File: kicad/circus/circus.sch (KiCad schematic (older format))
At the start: 119 parts, among them Q4 2N4093, Q5 2N4093, U6 MM5837, U8 LM348

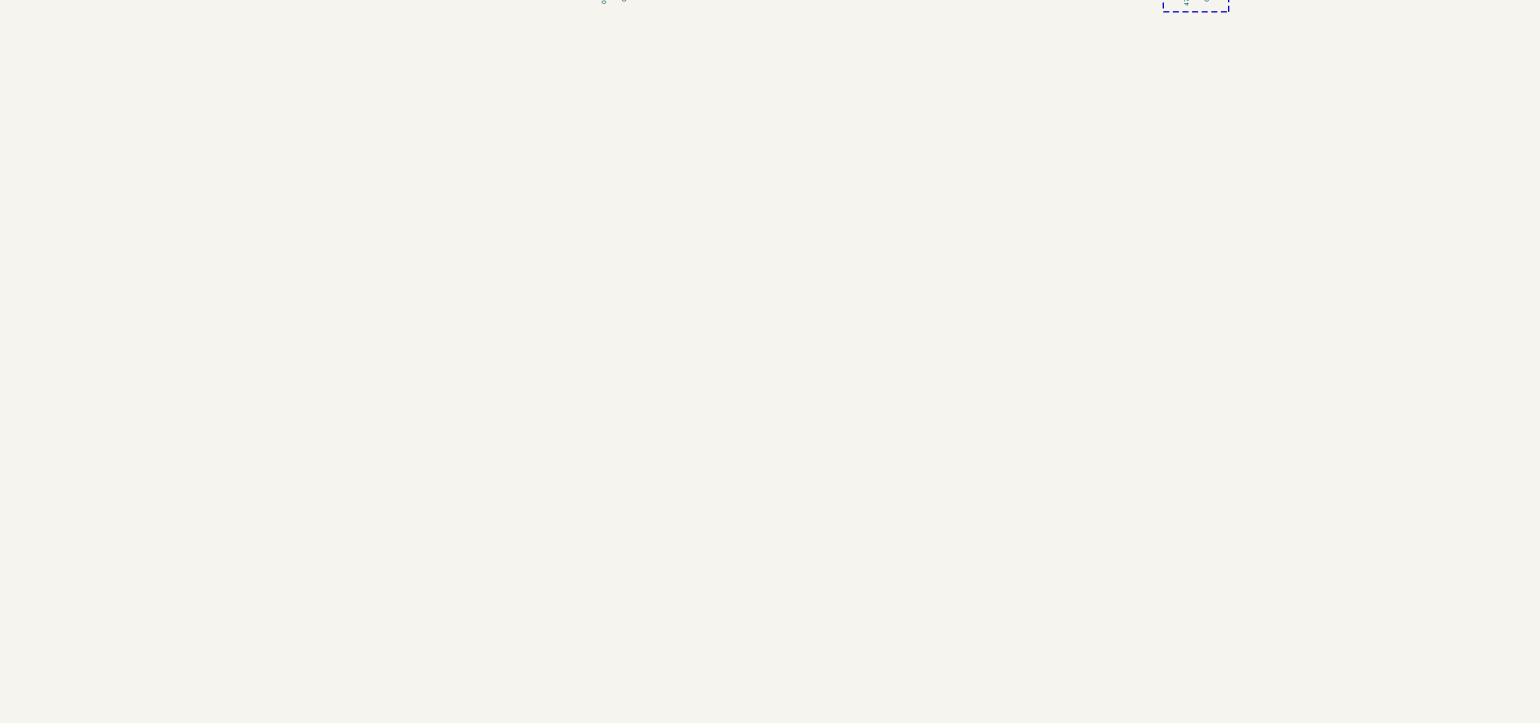
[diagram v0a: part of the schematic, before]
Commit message: The bear sound is now half-complete.
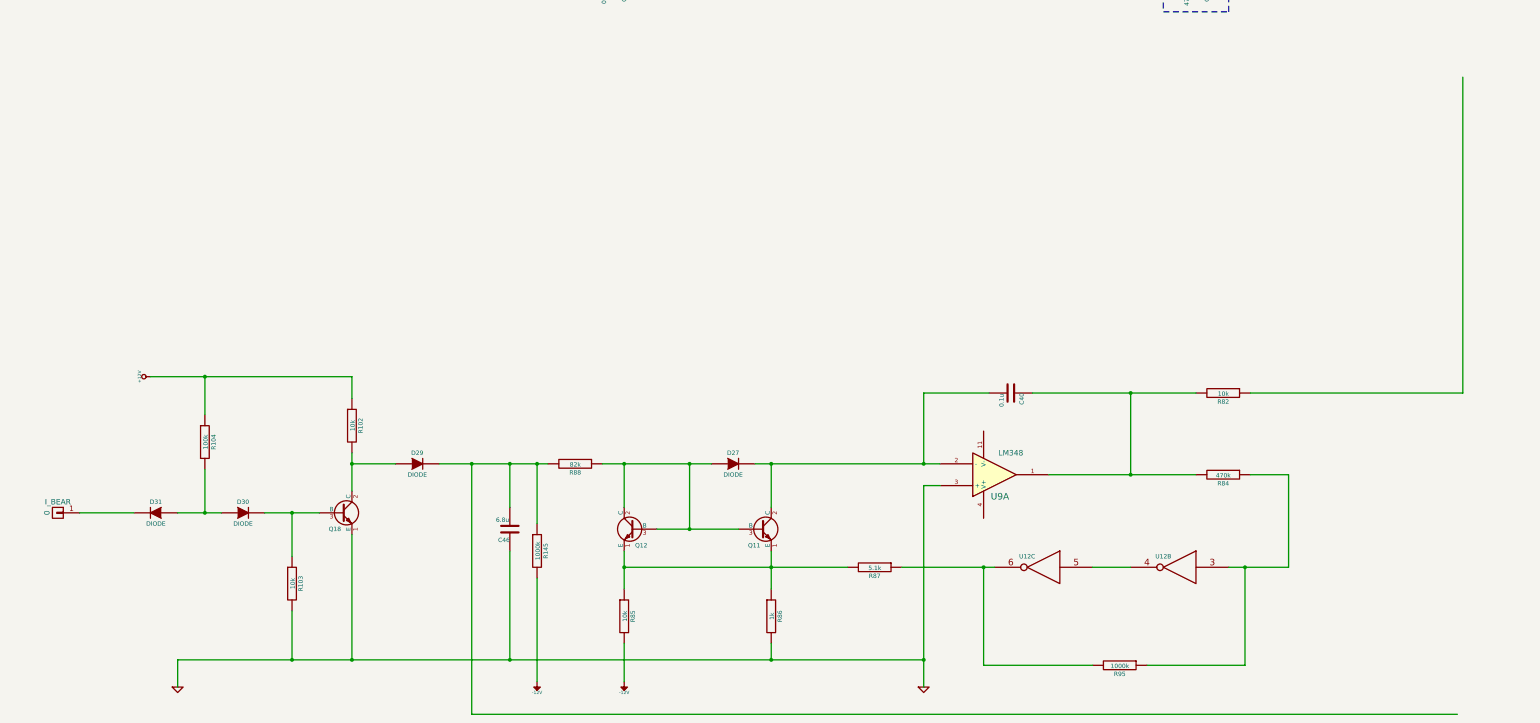
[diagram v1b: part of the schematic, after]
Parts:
- added C40: 0.1u, ~, symbol C
- added C46: 6.8u, ~, symbol C
- added D27, D29, D30, D31: DIODE, ~, symbol DIODE
- added I_BEAR: 0, symbol CONN_01X01
- added Q11, Q12, Q18: ~, symbol 2SC1941
- added R102, R103, R82, R85: 10k, ~, symbol R
- added R104: 100k, ~, symbol R
- added R145, R95: 1000k, ~, symbol R
- added R84: 470k, ~, symbol R
- added R86: 1k, ~, symbol R
- added R87: 5.1k, ~, symbol R
- added R88: 82k, ~, symbol R
- added U12: ~, ~, symbol 74HC04
- added U9: LM348, symbol LM324
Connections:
- net +12V: now also R102.1, R104.1
- net -12V: now also R145.2, R85.2
- net GND: now also C46.1, Q18.1 (E), R103.2, R86.2, U12.7 (GND), U12.7 (GND), U9.3 (+)
- net VCC: now also U12.14 (VCC), U12.14 (VCC)
- new net: D31.2 (K), I_BEAR.1 (P1)
- new net: D30.1 (A), D31.1 (A), R104.2
- new net: D30.2 (K), Q18.3 (B), R103.1
- new net: D29.1 (A), Q18.2 (C), R102.2
- new net: C46.2, D29.2 (K), R145.1, R88.2
- new net: Q11.1 (E), Q12.1 (E), R85.1, R86.1, R87.2
- new net: D27.1 (A), Q11.3 (B), Q12.2 (C), Q12.3 (B), R88.1
- new net: C40.2, D27.2 (K), Q11.2 (C), U9.2 (-)
- new net: R87.1, R95.2, U12.6
- new net: C40.1, R82.2, R84.2, U9.1
- new net: R84.1, R95.1, U12.3
- new net: U12.4, U12.5

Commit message: The Bear sound is complete.
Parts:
- added C39, C41, C45: 0.1u, ~, symbol C
- added C44: 0.0047u, ~, symbol C
- added D28: DIODE, ~, symbol DIODE
- added Q10, Q9: ~, symbol 2SC1941
- added R100, R94: 1000k, ~, symbol R
- added R101, R92: 470k, ~, symbol R
- added R76: 1k, ~, symbol R
- added R77, R83: 10k, ~, symbol R
- added R89, R90: 47k, ~, symbol R
- added R91: 33k, ~, symbol R
- added R93: 5.1k, ~, symbol R
- added unit 5 of U12
- added unit 4 of U12
- added unit 6 of U12
- added unit 1 of U12
- added unit 2 of U9
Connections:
- net -12V: now also R77.1
- net GND: now also R76.1, U12.7 (GND), U12.7 (GND), U12.7 (GND), U12.7 (GND), U9.5 (+)
- net VCC: now also U12.14 (VCC), U12.14 (VCC), U12.14 (VCC), U12.14 (VCC)
- net at R13.1, R27.1, R36.1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: now also R91.1
- net at C46.2, D29.2 (K), R145.1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: now also R101.2, R89.2
- net at R82.1: now also C39.1, R83.2
- new net: C39.2, R91.2
- new net: C41.1, R83.1, R92.1, U9.7
- new net: C44.2, R100.2, R101.1, U12.11
- new net: D28.1 (A), Q10.2 (C), Q10.3 (B), Q9.3 (B), R89.1, R90.1
- new net: R100.1, U12.10, U12.9
- new net: C44.1, C45.1, U12.8
- new net: C45.2, R90.2
- new net: C41.2, D28.2 (K), U9.6 (-)
- new net: Q10.1 (E), Q9.1 (E), R76.2, R77.2
- new net: Q9.2 (C), R93.1
- new net: R92.2, R94.1, U12.1
- new net: R93.2, R94.2, U12.12
- new net: U12.13, U12.2
